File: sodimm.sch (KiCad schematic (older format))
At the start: 3 parts, among them J5 2309409-1

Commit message: Replace SO-DIMM DDR4 to SO-DIMM DDR3 connector
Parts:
- removed J5: 2309409-1, lpddr4-test-board-footprints:TE_2309409-1, symbol lpddr4-test-board:2309409-1
- added J? (x2): ddr3-sodimm-slot-2-2013289-2, antmicro-footprints:TE_2-2013289-2, symbol antmicroMemoryConnectorsPCCardSockets:ddr3-sodimm-slot-2-2013289-2
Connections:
- net labels removed: BA0, BA1, BG0, BG1, CB0\NC, CB1\NC, CB2\NC, CB3\NC, CB4\NC, CB5\NC, CB6\NC, CB7\NC, DM4_n\DBI4_n, DM5_n\DBI5_n, DM6_n\DBI6_n, DM7_n\DBI_n, DM8_n\DBI_n\NC, DQ32, DQ33, DQ34, DQ35, DQ36, DQ37, DQ38, DQ39, DQ40, DQ41, DQ42, DQ43, DQ44, DQ45, DQ46, DQ47, DQ48, DQ49, DQ50, DQ51, DQ52, DQ53, DQ54, DQ55, DQ56, DQ57, DQ58, DQ59, DQ60, DQ61, DQ62, DQ63, DQS4_c, DQS4_t, DQS5_c, DQS5_t, DQS6_c, DQS6_t, DQS7_c, DQS7_t, DQS8_c\NC, DQS8_t\NC
- wire segments 379 -> 248
- no-connect marks 0 -> 53
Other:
- note added: "TODO: Decide what about this signals"

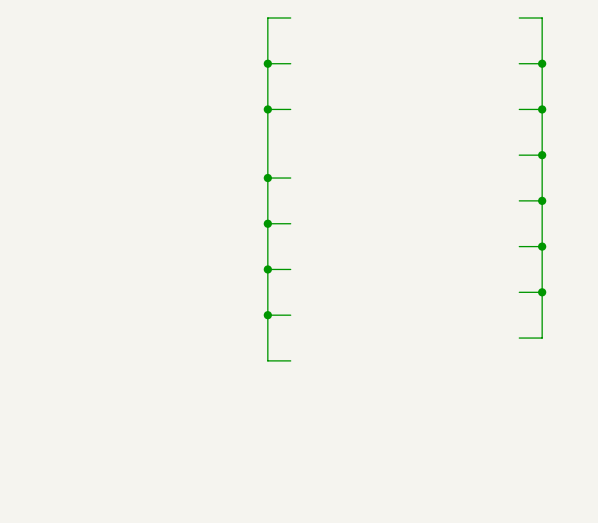
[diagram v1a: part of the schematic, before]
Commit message: Cleanup
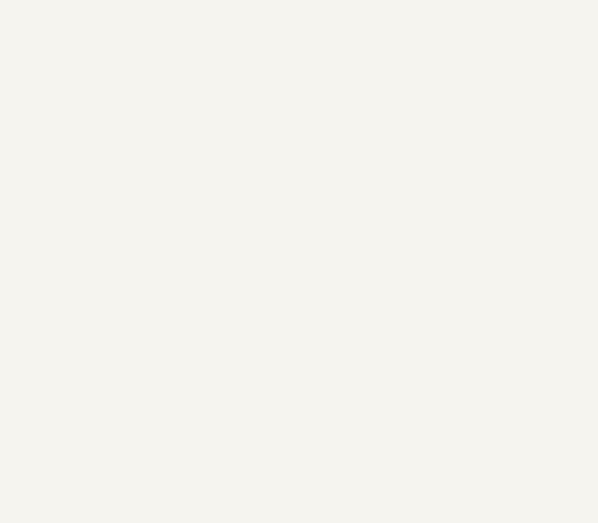
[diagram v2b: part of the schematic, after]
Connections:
- wire segments 248 -> 218
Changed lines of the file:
@@
 Comment4 ""
 $EndDescr
-Wire Wire Line
-	12725 -5950 12625 -5950
-Wire Wire Line
-	12725 -5750 12625 -5750
-Wire Wire Line
-	12725 -6550 12625 -6550
-Wire Wire Line
-	12725 -6350 12625 -6350
-Wire Wire Line
-	12725 -6150 12625 -6150
-Wire Wire Line
-	12725 -7250 12625 -7250
-Wire Wire Line
-	12725 -7050 12625 -7050
-Wire Wire Line
-	12725 -6850 12625 -6850
-Wire Wire Line
-	13825 -7250 13725 -7250
-Wire Wire Line
-	13825 -7050 13725 -7050
-Wire Wire Line
-	13825 -6850 13725 -6850
-Wire Wire Line
-	13825 -6650 13725 -6650
-Wire Wire Line
-	13825 -6450 13725 -6450
-Wire Wire Line
-	13825 -6250 13725 -6250
-Wire Wire Line
-	13825 -6050 13725 -6050
-Wire Wire Line
-	13825 -5850 13725 -5850
-Wire Wire Line
-	12625 -7250 12625 -7050
-Connection ~ 12625 -7050
-Wire Wire Line
-	12625 -7050 12625 -6850
-Connection ~ 12625 -6850
-Wire Wire Line
-	12625 -6850 12625 -6550
-Connection ~ 12625 -6550
-Wire Wire Line
-	12625 -6550 12625 -6350
-Connection ~ 12625 -6350
-Wire Wire Line
-	12625 -6350 12625 -6150
-Connection ~ 12625 -6150
-Wire Wire Line
-	12625 -6150 12625 -5950
-Connection ~ 12625 -5950
-Wire Wire Line
-	12625 -5950 12625 -5750
-Wire Wire Line
-	13825 -7250 13825 -7050
-Connection ~ 13825 -7050
-Wire Wire Line
-	13825 -7050 13825 -6850
-Connection ~ 13825 -6850
-Wire Wire Line
-	13825 -6850 13825 -6650
-Connection ~ 13825 -6650
-Wire Wire Line
-	13825 -6650 13825 -6450
-Connection ~ 13825 -6450
-Wire Wire Line
-	13825 -6450 13825 -6250
-Connection ~ 13825 -6250
-Wire Wire Line
-	13825 -6250 13825 -6050
-Connection ~ 13825 -6050
-Wire Wire Line
-	13825 -6050 13825 -5850
 $Comp
 L lpddr4-test-board:GND #PWR0230

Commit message: Add routing between FPGA and SO-DIMM WIP
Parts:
- gave numbers to parts that had none: 3
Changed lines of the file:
@@
 VDDQ
 $Comp
-L antmicroResistors0402:R_0R_0402 R?
+L antmicroResistors0402:R_0R_0402 R55
 U 1 1 606BFB95
 P 5325 9650
-F 0 "R?" H 5325 9725 60  0000 C CNN
+F 0 "R55" H 5325 9725 60  0000 C CNN
 F 1 "R_0R_0402" H 5325 9500 60  0001 C CNN
 F 2 "antmicro-footprints:0402-res" H 5525 9850 60  0001 L CNN
@@
 $EndComp
 $Comp
-L antmicroResistors0402:R_0R_0402 R?
+L antmicroResistors0402:R_0R_0402 R56
 U 1 1 606C1C63
 P 5325 9825
-F 0 "R?" H 5325 9900 60  0000 C CNN
+F 0 "R56" H 5325 9900 60  0000 C CNN
 F 1 "R_0R_0402" H 5325 9675 60  0001 C CNN
 F 2 "antmicro-footprints:0402-res" H 5525 10025 60  0001 L CNN
@@
 	5275 3300 5275 3600
 $Comp
-L lpddr4-test-board:GND #PWR?
+L lpddr4-test-board:GND #PWR0179
 U 1 1 60D2B1F7
 P 5275 7525
-F 0 "#PWR?" H 5275 7275 50  0001 C CNN
+F 0 "#PWR0179" H 5275 7275 50  0001 C CNN
 F 1 "GND" H 5280 7352 50  0000 C CNN
 F 2 "" H 5275 7525 50  0001 C CNN
@@
 $EndComp
 $Comp
-L antmicroMemoryConnectorsPCCardSockets:ddr3-sodimm-slot-2-2013289-2 J?
+L antmicroMemoryConnectorsPCCardSockets:ddr3-sodimm-slot-2-2013289-2 J9
 U 1 1 60D77CED
 P 4350 5100
-F 0 "J?" H 4350 7267 50  0000 C CNN
+F 0 "J9" H 4350 7267 50  0000 C CNN
 F 1 "ddr3-sodimm-slot-2-2013289-2" H 4350 7176 50  0000 C CNN
 F 2 "antmicro-footprints:TE_2-2013289-2" H 4350 5100 50  0001 L BNN
@@
 $EndComp
 $Comp
-L antmicroMemoryConnectorsPCCardSockets:ddr3-sodimm-slot-2-2013289-2 J?
+L antmicroMemoryConnectorsPCCardSockets:ddr3-sodimm-slot-2-2013289-2 J9
 U 2 1 60D7BA8A
 P 11175 5775
-F 0 "J?" H 11175 9442 50  0000 C CNN
+F 0 "J9" H 11175 9442 50  0000 C CNN
 F 1 "ddr3-sodimm-slot-2-2013289-2" H 11175 9351 50  0000 C CNN
 F 2 "antmicro-footprints:TE_2-2013289-2" H 11175 5775 50  0001 L BNN
@@
 VDD1
 $Comp
-L lpddr4-test-board:GND #PWR?
+L lpddr4-test-board:GND #PWR0180
 U 1 1 65590887
 P 10250 9400
-F 0 "#PWR?" H 10250 9150 50  0001 C CNN
+F 0 "#PWR0180" H 10250 9150 50  0001 C CNN
 F 1 "GND" H 10255 9227 50  0000 C CNN
 F 2 "" H 10250 9400 50  0001 C CNN
@@
 $EndComp
 $Comp
-L lpddr4-test-board:GND #PWR?
+L lpddr4-test-board:GND #PWR0200
 U 1 1 655A29FD
 P 12100 9400
-F 0 "#PWR?" H 12100 9150 50  0001 C CNN
+F 0 "#PWR0200" H 12100 9150 50  0001 C CNN
 F 1 "GND" H 12105 9227 50  0000 C CNN
 F 2 "" H 12100 9400 50  0001 C CNN

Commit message: Rebuild connections to fit lpddr4 module (WIP)
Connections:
- net labels added: CK0_N, CK0_P, CK1_N, CK1_P, CKE0_A, CKE0_B, CS0_N_B, DQS0_N, DQS0_P, DQS1_N, DQS1_P, DQS2_N, DQS2_P, DQS3_N, DQS3_P
- net labels removed: CK0_c, CK0_t, CK1_c\NF, CK1_t\NF, CKE0, CKE1\NC, CS1_n\NC, DQS0_c, DQS0_t, DQS1_c, DQS1_t, DQS2_c, DQS2_t, DQS3_c, DQS3_t
- wire segments 218 -> 246
- no-connect marks 53 -> 0
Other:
- note added: "TODO: Decide what about this signals\n(not included in lpddr4 pinout doc)"
- note added: "TODO: Decide where to put VCC"
- note removed: "TODO: Decide what about this signals"

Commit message: Add LPDDR4 routing and equalize traces - WIP
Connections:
- net labels added: CA0_A, CA0_B, CA1_A, CA1_B, CA2_A, CA2_B, CA3_A, CA3_B, CA4_A, CA4_B, CA5_A, CA5_B
- net labels removed: A0, A1, A10\AP, A11, A12, A13, A2, A3, A4, A5, A6, A7, A8, A9, ACT_n, ALERT_n, C0\CS2_n\NC, C1\CS3_n\NC, CAS_n\A15, EVENT_n\NF, PARITY, RAS_n\A16, SA0, SA1, SA2, SCL, SDA, VDDSPD, VPP, VREFCA, VTT, WE_n\A14
- wire segments 246 -> 243
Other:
- note removed: "TODO: Decide what about this signals\n(not included in lpddr4 pinout doc)"
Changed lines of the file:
@@
 	1    0    0    -1
 $EndComp
-Text GLabel 16950 6875 0    50   Input ~ 0
+Text GLabel 5725 5300 2    50   Input ~ 0
 VDDQ
-Text GLabel 17000 6675 0    50   Input ~ 0
+Text GLabel 3000 5300 0    50   Input ~ 0
 VDDQ
-Text GLabel 17075 5000 0    50   Input ~ 0
-VDDSPD
 Wire Wire Line
 	11875 6275 12575 6275
@@
 Wire Wire Line
 	10475 2875 9775 2875
-Wire Wire Line
-	17450 5825 16750 5825
-Wire Wire Line
-	17450 5725 16750 5725
-Wire Wire Line
-	17450 5525 16750 5525
 Text GLabel 9775 5575 0    50   Input ~ 0
 DQ5
@@
 CKE0_A
 Text GLabel 9775 2875 0    50   Input ~ 0
-A12
-Text GLabel 16750 5825 0    50   Input ~ 0
-A9
-Text GLabel 16750 5725 0    50   Input ~ 0
-A8
-Text GLabel 16750 5525 0    50   Input ~ 0
-A6
+CA2_B
 Wire Wire Line
 	10475 7275 9775 7275
@@
 Wire Wire Line
 	11875 2775 12575 2775
-Wire Wire Line
-	17600 7750 16900 7750
-Wire Wire Line
-	17375 7050 17075 7050
-Wire Wire Line
-	16475 8550 17175 8550
 Text GLabel 9775 7275 0    50   Input ~ 0
-A1
+CA1_A
 Text GLabel 12575 4975 2    50   Input ~ 0
 CK0_P
 Text GLabel 12575 5075 2    50   Input ~ 0
 CK0_N
-Text GLabel 16875 3925 2    50   Input ~ 0
-PARITY
 Text GLabel 12575 7275 2    50   Input ~ 0
 CS0_n
-Text GLabel 12575 2775 2    50   Input ~ 0
-WE_n\A14
-Text GLabel 16900 7750 0    50   Input ~ 0
-ODT0
 Text GLabel 12575 3075 2    50   Input ~ 0
 CS0_N_B
-Text GLabel 17075 7050 0    50   Input ~ 0
-ODT1\NC
-Text GLabel 16900 4375 2    50   Input ~ 0
-C1\CS3_n\NC
-Text GLabel 17175 8550 2    50   Input ~ 0
-SCL
-Text GLabel 17075 5100 0    50   Input ~ 0
-VPP
 Wire Wire Line
 	9775 5475 10475 5475
@@
 	12575 3275 11875 3275
 Wire Wire Line
-	17400 7925 16700 7925
-Wire Wire Line
 	12575 2975 11875 2975
 Wire Wire Line
 	9775 3075 10475 3075
 Wire Wire Line
-	16750 5625 17450 5625
-Wire Wire Line
 	12575 7675 11875 7675
 Wire Wire Line
@@
 	9775 7475 10475 7475
 Wire Wire Line
-	17175 8350 16475 8350
-Wire Wire Line
 	12575 5275 11875 5275
 Wire Wire Line
@@
 	9775 3175 10475 3175
 Wire Wire Line
-	17075 7600 17275 7600
-Wire Wire Line
 	12575 2675 11875 2675
 Wire Wire Line
 	9775 2775 10475 2775
-Wire Wire Line
-	17175 8450 16475 8450
-Wire Wire Line
-	16725 8050 17425 8050
-Wire Wire Line
-	16725 8250 17425 8250
 Text GLabel 12575 5975 2    50   Input ~ 0
 DQ0
@@
 Text GLabel 12575 3275 2    50   Input ~ 0
 DQ27
-Text GLabel 17400 7925 2    50   Input ~ 0
+Text GLabel 12575 7875 2    50   Input ~ 0
 RESET_n
-Text GLabel 16900 4625 2    50   Input ~ 0
-ACT_n
-Text GLabel 16900 4725 2    50   Input ~ 0
-ALERT_n
 Text GLabel 9775 3075 0    50   Input ~ 0
-A11
-Text GLabel 16750 5625 0    50   Input ~ 0
-A7
+CA1_B
 Text GLabel 12575 7675 2    50   Input ~ 0
-A5
+CA5_A
 Text GLabel 12575 7575 2    50   Input ~ 0
-A4
+CA4_A
 Text GLabel 9775 7475 0    50   Input ~ 0
-A2
-Text GLabel 17175 8350 2    50   Input ~ 0
-EVENT_n\NF
+CA2_A
+Text GLabel 12575 5375 2    50   Input ~ 0
+CK1_P
 Text GLabel 12575 5275 2    50   Input ~ 0
-CK1_P
-Text GLabel 12575 5375 2    50   Input ~ 0
 CK1_N
 Text GLabel 9775 7175 0    50   Input ~ 0
-A0
+CA0_A
 Text GLabel 9775 3175 0    50   Input ~ 0
-A10\AP
-Text GLabel 17075 7600 0    50   Input ~ 0
-RAS_n\A16
-Text GLabel 12575 2675 2    50   Input ~ 0
-CAS_n\A15
+CA0_B
 Text GLabel 9775 2775 0    50   Input ~ 0
-A13
-Text GLabel 16900 4275 2    50   Input ~ 0
-C0\CS2_n\NC
-Text GLabel 16775 5200 2    50   Input ~ 0
-VREFCA
-Text GLabel 16900 4025 2    50   Input ~ 0
-SA2
-Text GLabel 17175 8450 2    50   Input ~ 0
-SDA
-Text GLabel 16725 8050 0    50   Input ~ 0
-SA0
-Text GLabel 16925 5300 2    50   Input ~ 0
-VTT
-Text GLabel 16725 8250 0    50   Input ~ 0
-SA1
+CA3_B
 Wire Wire Line
 	10475 7575 9775 7575
 Text GLabel 9775 7575 0    50   Input ~ 0
-A3
+CA3_A
 Text GLabel 12575 2975 2    50   Input ~ 0
 CKE0_B
@@
 Text Notes 7375 1325 0    118  ~ 24
 SODIMM connector
-Text GLabel 16725 7175 0    50   Input ~ 0
+Text GLabel 3000 5175 0    50   Input ~ 0
 VDD1V8
 Text GLabel 4550 9625 2    50   Input ~ 0
@@
 Text GLabel 4550 9800 2    50   Input ~ 0
 VDD0V6
-Text Notes 16700 6250 0    50   ~ 0
+Text Notes 6025 5075 2    50   ~ 0
 VDD1
-Text GLabel 17000 6375 0    50   Input ~ 0
+Text GLabel 5725 5175 2    50   Input ~ 0
 VDD1V8
-Text GLabel 2400 2975 0    50   Input ~ 0
+Text GLabel 3100 2625 0    50   Input ~ 0
 VDD1V1
-Text GLabel 6000 3025 2    50   Input ~ 0
+Text GLabel 5575 2600 2    50   Input ~ 0
 VDD1V1
-Text Notes 2125 2825 0    50   ~ 0
+Text Notes 2825 2475 0    50   ~ 0
 VDD2\n
 Text GLabel 3925 9625 0    50   Input ~ 0
@@
 	5275 7000 5275 7525
 Wire Wire Line
-	2400 2975 2400 3650
-Connection ~ 2400 3950
-Wire Wire Line
-	2400 3950 2400 4250
-Wire Wire Line
-	2400 3950 2600 3950
-Wire Wire Line
-	2600 4250 2400 4250
-Connection ~ 2400 4250
-Wire Wire Line
-	2400 4250 2400 4550
-Wire Wire Line
-	17000 6675 17375 6675
-Wire Wire Line
-	17375 6375 17000 6375
-Wire Wire Line
-	2600 5450 2400 5450
-Wire Wire Line
-	2600 5150 2400 5150
-Connection ~ 2400 5150
-Wire Wire Line
-	2400 5150 2400 5450
-Wire Wire Line
-	2600 4850 2400 4850
-Connection ~ 2400 4850
-Wire Wire Line
-	2400 4850 2400 5150
-Wire Wire Line
-	2600 4550 2400 4550
-Connection ~ 2400 4550
-Wire Wire Line
-	2400 4550 2400 4850
-Wire Wire Line
-	2600 3650 2400 3650
-Connection ~ 2400 3650
-Wire Wire Line
-	2400 3650 2400 3950
-Wire Wire Line
-	6000 3025 6000 3700
-Connection ~ 6000 4000
-Wire Wire Line
-	6000 4000 6000 4300
-Wire Wire Line
-	6000 4000 5800 4000
-Wire Wire Line
-	5800 4300 6000 4300
-Connection ~ 6000 4300
-Wire Wire Line
-	6000 4300 6000 4600
-Wire Wire Line
-	16950 6875 17375 6875
-Wire Wire Line
-	17375 7175 16950 7175
-Wire Wire Line
-	17425 7475 16950 7475
-Wire Wire Line
-	16950 7475 16950 7175
-Wire Wire Line
-	5800 5200 6000 5200
-Wire Wire Line
-	5800 4900 6000 4900
-Connection ~ 6000 4900
-Wire Wire Line
-	6000 4900 6000 5200
-Wire Wire Line
-	5800 4600 6000 4600
-Connection ~ 6000 4600
-Wire Wire Line
-	6000 4600 6000 4900
-Wire Wire Line
-	5800 3700 6000 3700
-Connection ~ 6000 3700
-Wire Wire Line
-	6000 3700 6000 4000
+	3100 2625 3100 3300
+Connection ~ 3100 3600
+Wire Wire Line
+	3650 3800 3100 3800
+Wire Wire Line
+	3650 4300 3100 4300
+Wire Wire Line
+	3650 4100 3100 4100
+Wire Wire Line
+	3650 4000 3100 4000
+Connection ~ 3100 3300
+Wire Wire Line
+	3100 3300 3100 3500
+Wire Wire Line
+	5575 3500 5050 3500
+Wire Wire Line
+	5050 3700 5575 3700
+Wire Wire Line
+	5050 4100 5575 4100
+Wire Wire Line
+	5050 4000 5575 4000
+Wire Wire Line
+	5050 3800 5575 3800
+Wire Wire Line
+	5050 3400 5575 3400
 Wire Wire Line
 	11875 5475 12100 5475
 Wire Wire Line
 	10475 5175 10250 5175
-Text Notes 6125 2900 0    50   ~ 0
+Text Notes 5700 2475 0    50   ~ 0
 VDD2\n
-Wire Wire Line
-	16950 7175 16725 7175
-Connection ~ 16950 7175
-Text Notes 16625 7325 2    50   ~ 0
+Text Notes 2875 5100 2    50   ~ 0
 VDD1
 $Comp
@@
 	1    0    0    -1
 $EndComp
-Wire Notes Line
-	16150 3375 17800 3375
-Text Notes 16150 3550 0    50   ~ 0
-TODO: Decide what about this signals\n(not included in lpddr4 pinout doc)
 Text GLabel 12575 6475 2    50   Input ~ 0
 DQS1_N
@@
 Wire Notes Line
 	17825 8800 16200 8800
-Wire Notes Line
-	17800 3375 17825 8825
 Text Notes 3725 2325 0    50   ~ 0
 TODO: Decide where to put VCC
@@
 Wire Wire Line
 	12100 7775 12100 9400
+Text GLabel 9775 7875 0    50   Input ~ 0
+ODT1\NC
+Text GLabel 9775 7775 0    50   Input ~ 0
+ODT0
+Text GLabel 12575 2675 2    50   Input ~ 0
+CA5_B
+Text GLabel 12575 2775 2    50   Input ~ 0
+CA4_B
+Wire Wire Line
+	12575 7875 11875 7875
+Wire Wire Line
+	9775 7775 10475 7775
+Wire Wire Line
+	10475 7875 9775 7875
+Wire Wire Line
+	3100 3300 3650 3300
+Wire Wire Line
+	3100 3500 3650 3500
+Connection ~ 3100 3500
+Wire Wire Line
+	3100 3500 3100 3600
+Wire Wire Line
+	3100 3600 3650 3600
+Connection ~ 3100 3800
+Wire Wire Line
+	3100 3800 3100 4000
+Wire Wire Line
+	3100 3600 3100 3800
+Connection ~ 3100 4000
+Wire Wire Line
+	3100 4000 3100 4100
+Connection ~ 3100 4100
+Wire Wire Line
+	3100 4100 3100 4300
+Connection ~ 3100 4300
+Wire Wire Line
+	3100 4300 3100 4400
+Connection ~ 3100 4400
+Wire Wire Line
+	3100 4400 3100 4600
+Wire Wire Line
+	3100 4400 3650 4400
+Wire Wire Line
+	5575 2600 5575 3400
+Connection ~ 5575 3400
+Wire Wire Line
+	5575 3400 5575 3500
+Connection ~ 5575 3500
+Wire Wire Line
+	5575 3500 5575 3700
+Connection ~ 5575 3700
+Wire Wire Line
+	5575 3700 5575 3800
+Connection ~ 5575 3800
+Wire Wire Line
+	5575 3800 5575 4000
+Connection ~ 5575 4000
+Wire Wire Line
+	5575 4000 5575 4100
+Connection ~ 5575 4100
+Wire Wire Line
+	5575 4100 5575 4300
+Wire Wire Line
+	5050 4300 5575 4300
+Connection ~ 5575 4300
+Wire Wire Line
+	5575 4300 5575 4400
+Wire Wire Line
+	5575 4400 5050 4400
+Connection ~ 5575 4400
+Wire Wire Line
+	5575 4400 5575 4600
+Wire Wire Line
+	5050 4600 5575 4600
+Connection ~ 5575 4600
+Wire Wire Line
+	5575 4600 5575 4700
+Wire Wire Line
+	5575 4700 5050 4700
+Wire Wire Line
+	3650 4600 3100 4600
+Connection ~ 3100 4600
+Wire Wire Line
+	3100 4600 3100 4700
+Wire Wire Line
+	3650 4700 3100 4700
 $EndSCHEMATC

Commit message: Add LPDDR4 routing with equalized traces - WIP
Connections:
- net labels added: CS0_N_A, ODT1
- net labels removed: CS0_n, ODT1\NC
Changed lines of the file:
@@
 CK0_N
 Text GLabel 12575 7275 2    50   Input ~ 0
-CS0_n
+CS0_N_A
 Text GLabel 12575 3075 2    50   Input ~ 0
 CS0_N_B
@@
 	12100 7775 12100 9400
 Text GLabel 9775 7875 0    50   Input ~ 0
-ODT1\NC
+ODT1
 Text GLabel 9775 7775 0    50   Input ~ 0
 ODT0
